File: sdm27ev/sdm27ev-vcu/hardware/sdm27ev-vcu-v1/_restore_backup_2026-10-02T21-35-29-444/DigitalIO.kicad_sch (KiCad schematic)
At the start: 28 parts, among them IC17 TPD4E05U06QDQARQ1, IC18 TPD4E05U06QDQARQ1, IC19 TPD4E05U06QDQARQ1, U2 TBD62783AFNG_EL, U8 LM2903BIPWR, U9 LM2903BIPWR

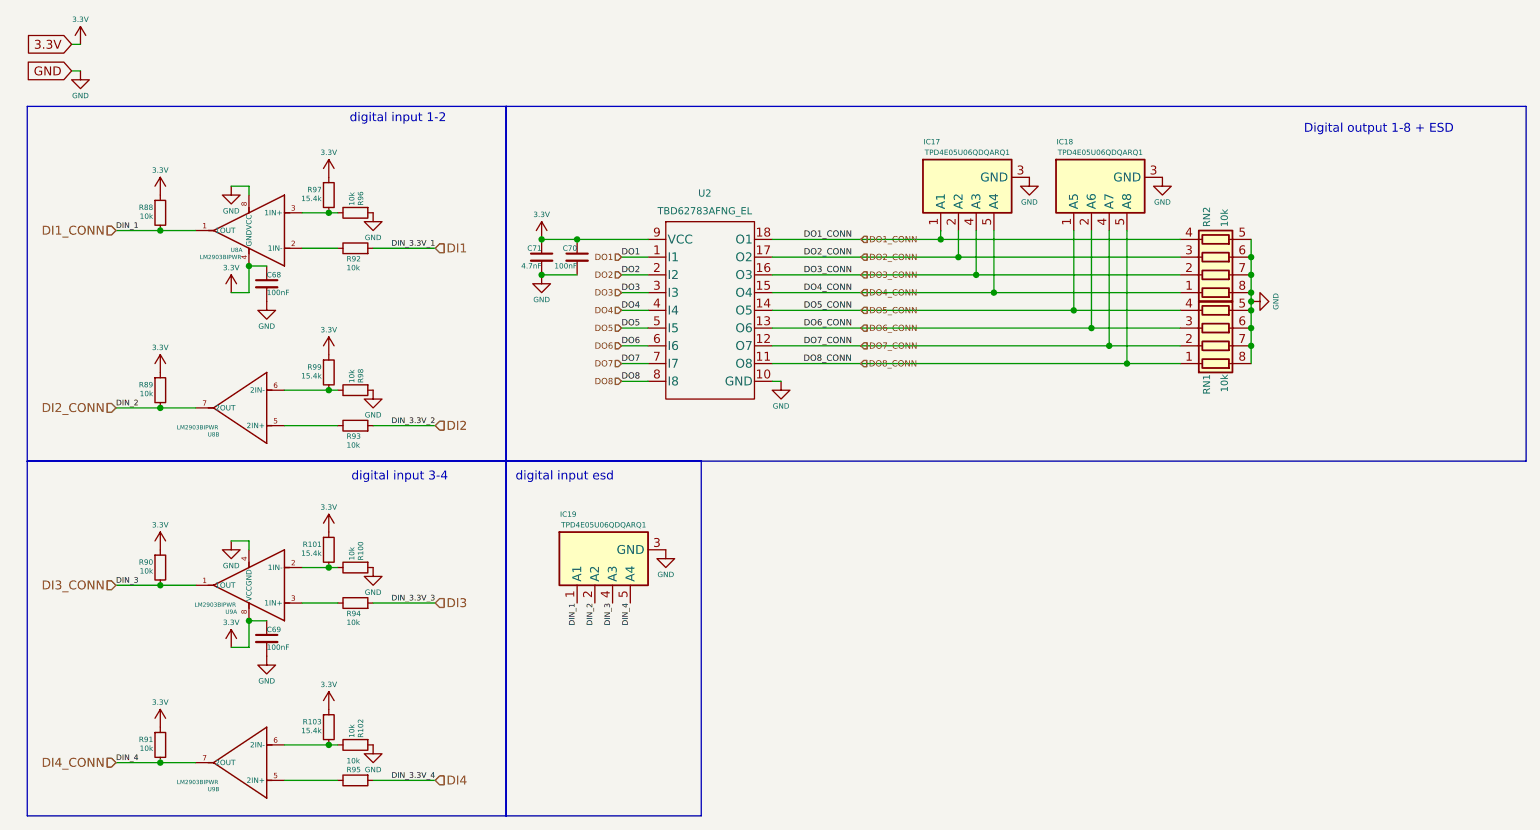
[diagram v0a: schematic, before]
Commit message: SDM27 EV VCU Final SCH + docs edit
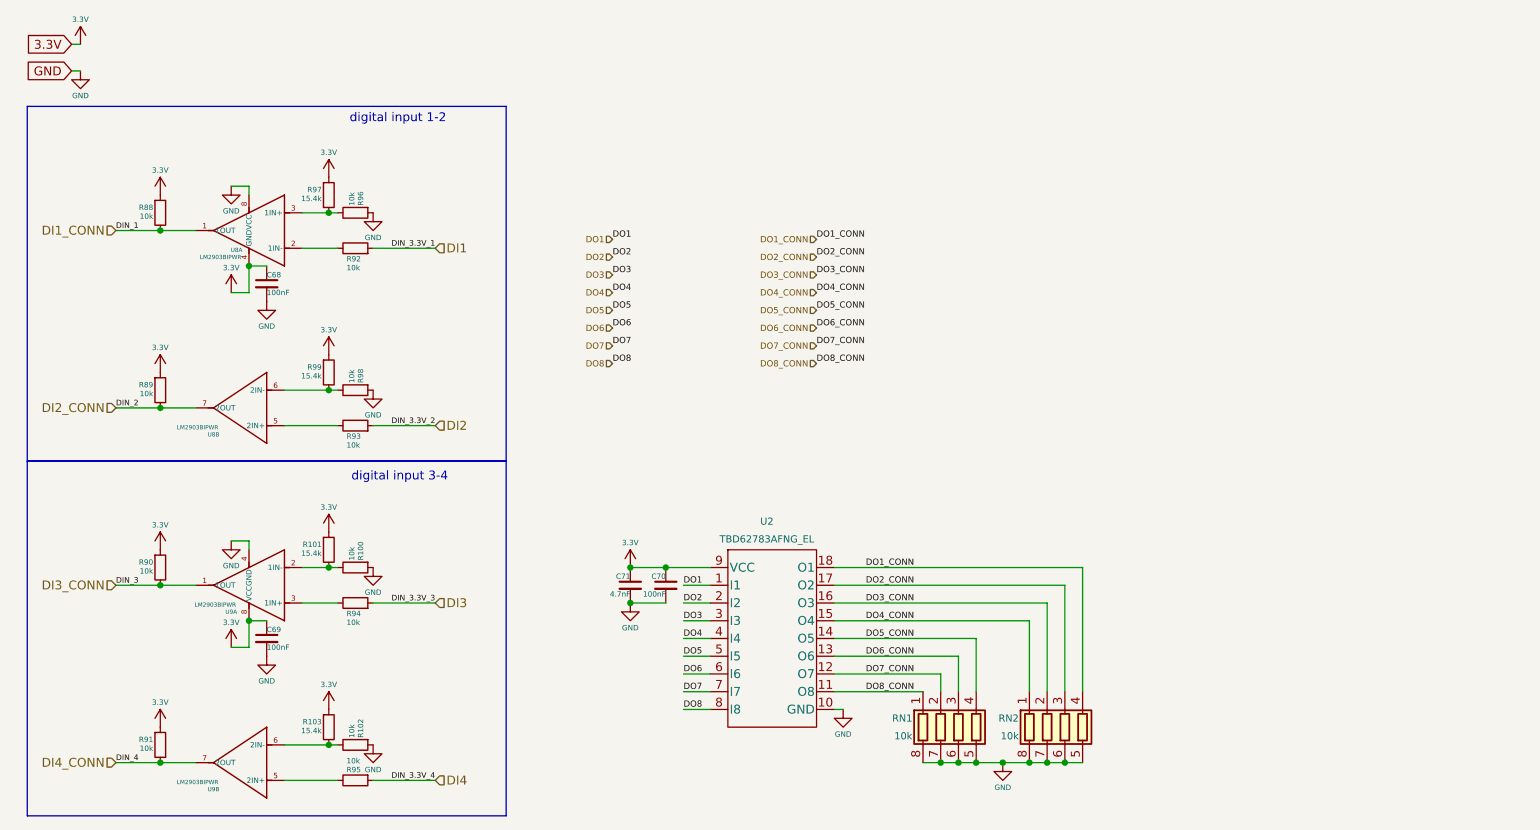
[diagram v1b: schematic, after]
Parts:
- removed IC17, IC18, IC19: TPD4E05U06QDQARQ1, DQA(R-PUSON-N10), symbol SDM_EV:TPD4E05U06QDQARQ1
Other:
- note removed: "Digital output 1-8 + ESD"
- note removed: "digital input esd"
- moved on the sheet: C70, C71, RN1, RN2, U2
